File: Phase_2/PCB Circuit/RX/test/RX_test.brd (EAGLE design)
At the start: 160 x 100 mm, 12 parts

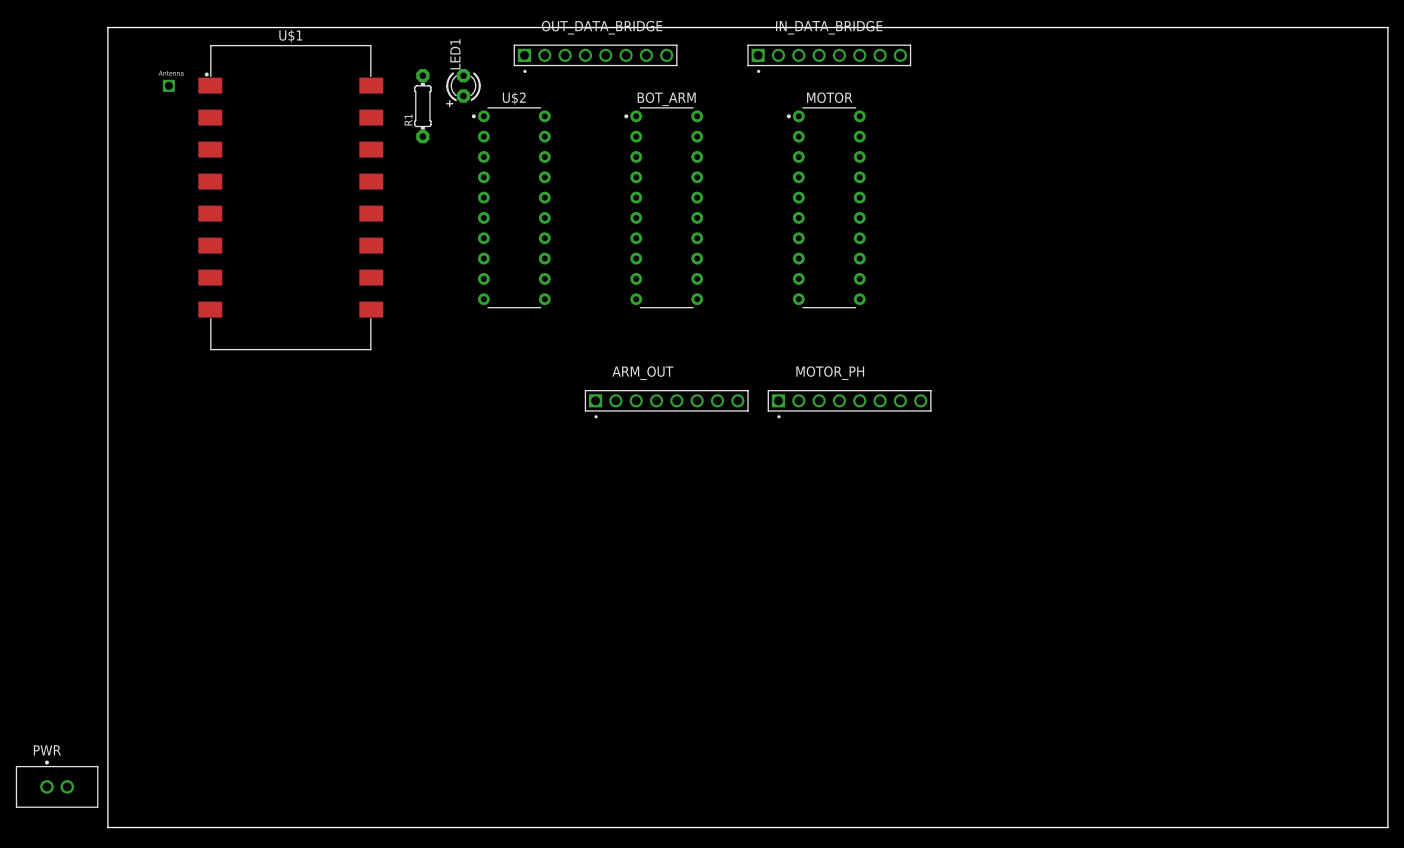
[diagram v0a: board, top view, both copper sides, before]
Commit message: 5+4
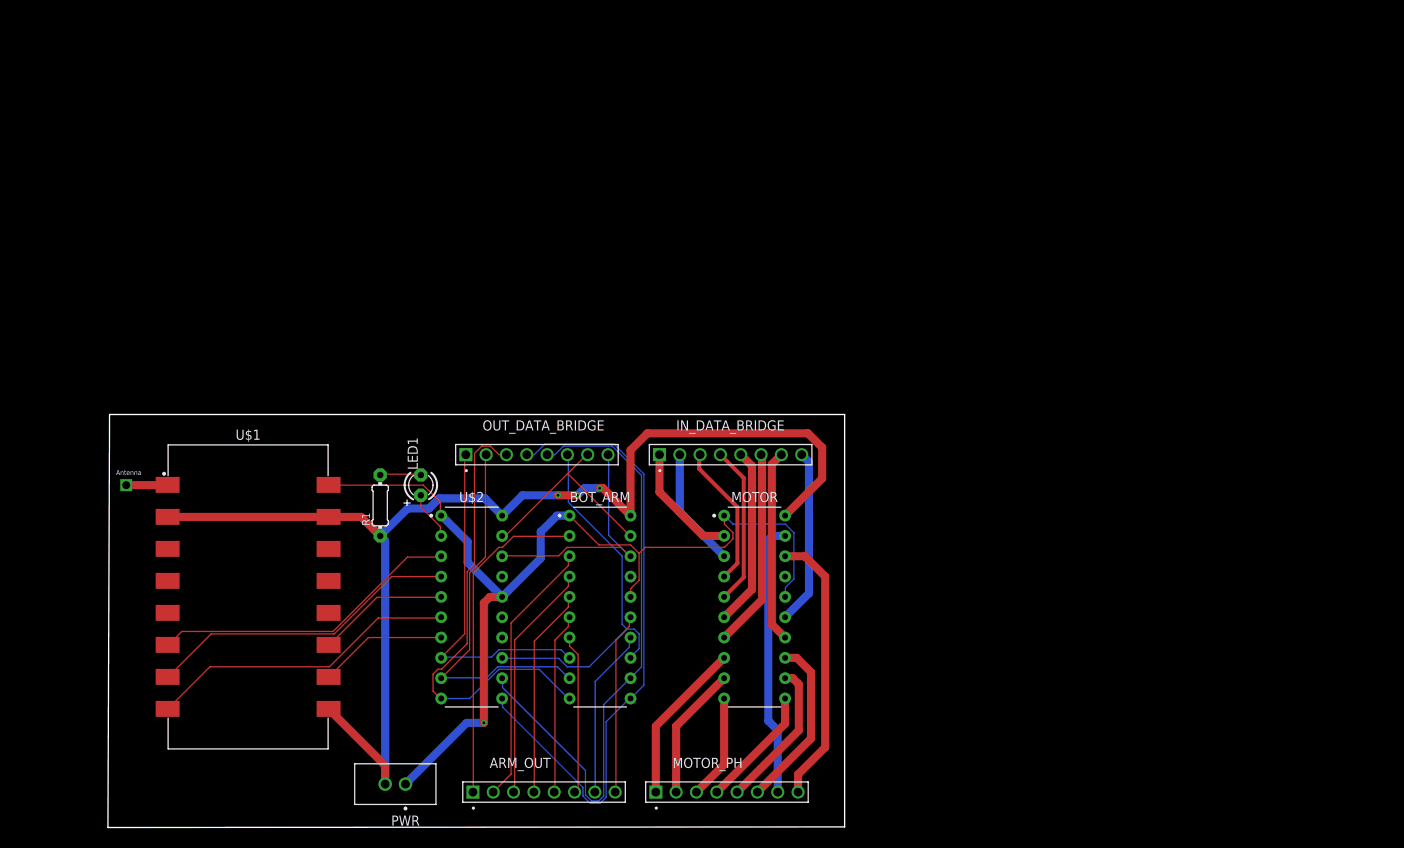
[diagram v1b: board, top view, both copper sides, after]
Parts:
- moved IN_DATA_BRIDGE 51.4 mm to (77.8, 46.6)
- moved ARM_OUT 51.3 mm to (54.5, 4.43)
- moved MOTOR_PH 51.3 mm to (77.4, 4.43)
- moved MOTOR 50.8 mm to (80.8, 27.6)
- moved BOT_ARM 50.6 mm to (61.5, 27.6)
- moved OUT_DATA_BRIDGE 50.4 mm to (53.6, 46.6)
- moved R1 50.2 mm to (34.0, 40.3)
- moved U$2 50.2 mm to (45.5, 27.6)
- moved LED1 50.2 mm to (39.1, 42.8)
- moved U$1 50.2 mm to (17.5, 28.8)
- moved U$4 50.2 mm to (2.29, 42.8)
- moved PWR 44.8 mm to (37.2, 5.43), turned to 180 degrees
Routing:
- net GND: track 0.00 -> 157.4 mm, vias 0 -> 3
- net VCC: track 0.00 -> 125.9 mm, vias 0 -> 1
- net PORT3: track 0.00 -> 79.2 mm
- net PORT4: track 0.00 -> 77.6 mm
- net PORT2: track 0.00 -> 57.4 mm
- net PORT5: track 0.00 -> 48.2 mm
- net PORT1: track 0.00 -> 47.5 mm
- net PORT0: track 0.00 -> 43.6 mm
- net OPORT0: track 0.00 -> 41.3 mm
- net N$7: track 0.00 -> 39.4 mm
- net N$8: track 0.00 -> 38.9 mm
- net N$6: track 0.00 -> 38.8 mm
- net MPORT7: track 0.00 -> 34.4 mm
- net MPORT6: track 0.00 -> 34.3 mm
- net OPORT1: track 0.00 -> 33.4 mm
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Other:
- board size 160 x 100 mm -> 92.1 x 51.6 mm
